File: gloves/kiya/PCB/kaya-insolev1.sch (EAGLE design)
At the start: 16 parts, among them U1 LSM9DS1, U2 MCP73832T-2ACI/OT

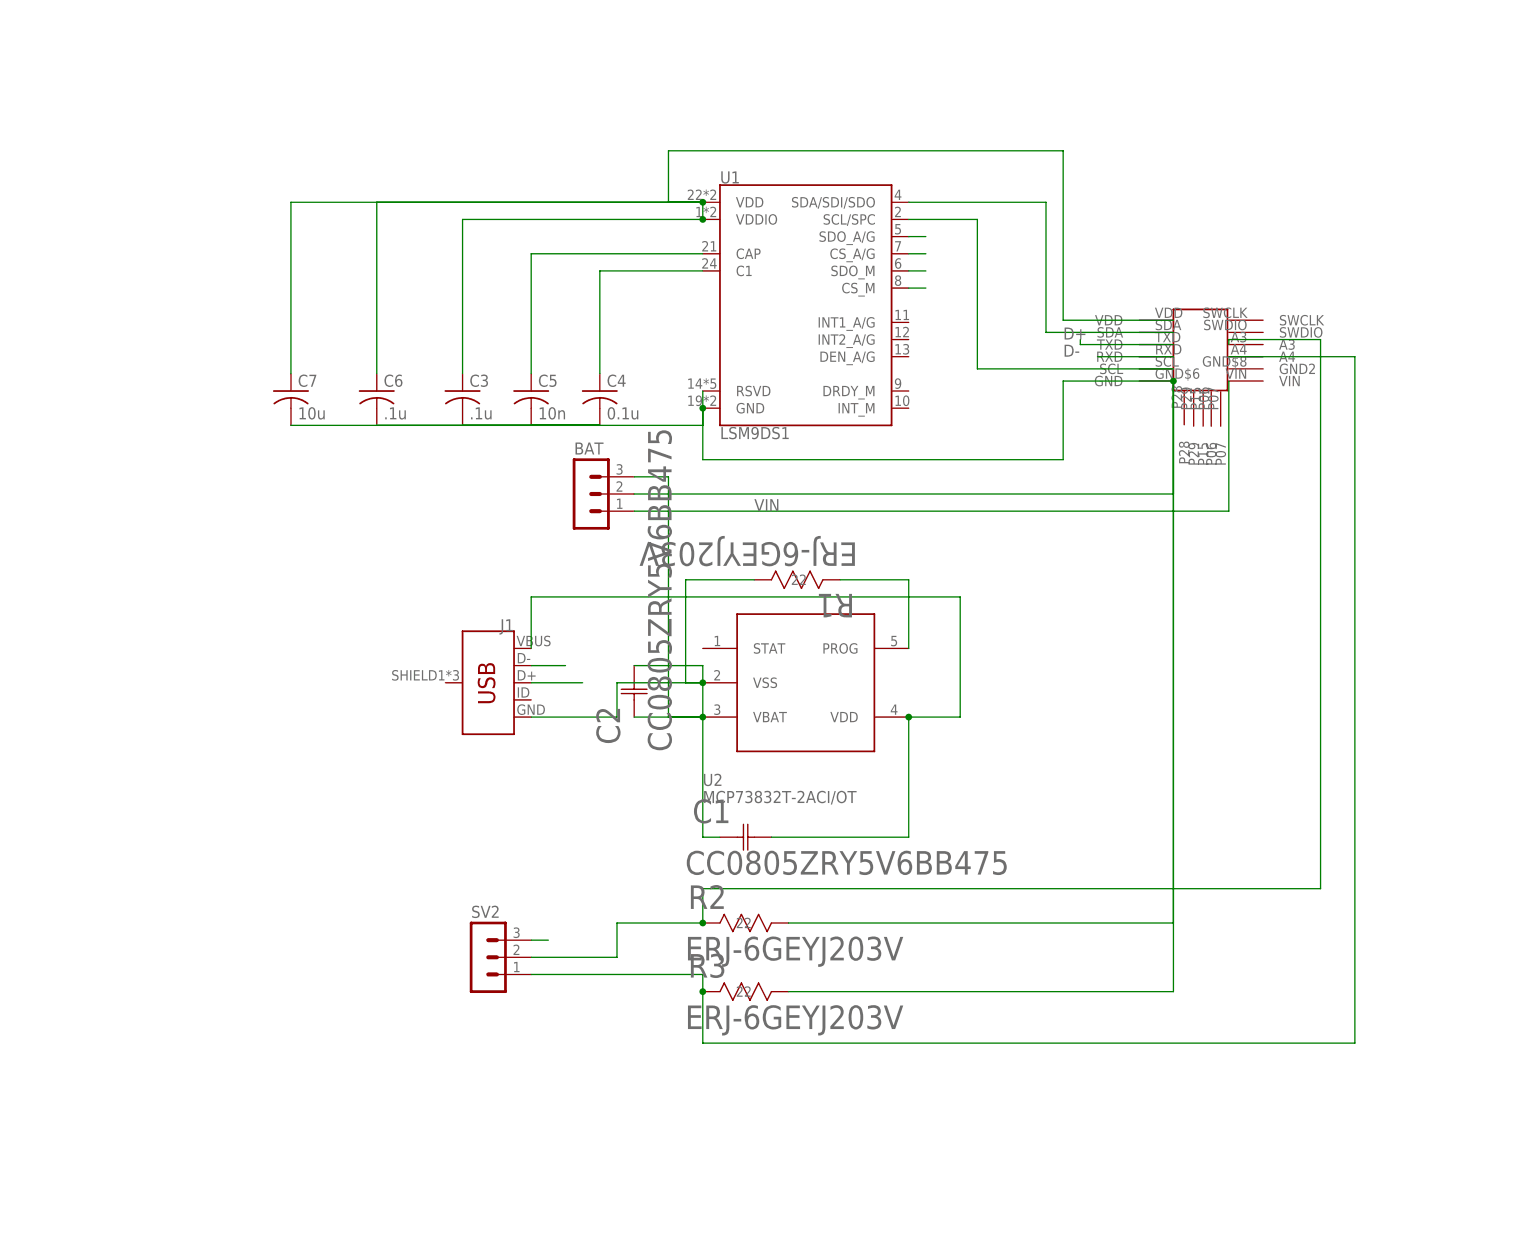
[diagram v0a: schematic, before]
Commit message: PCB v1
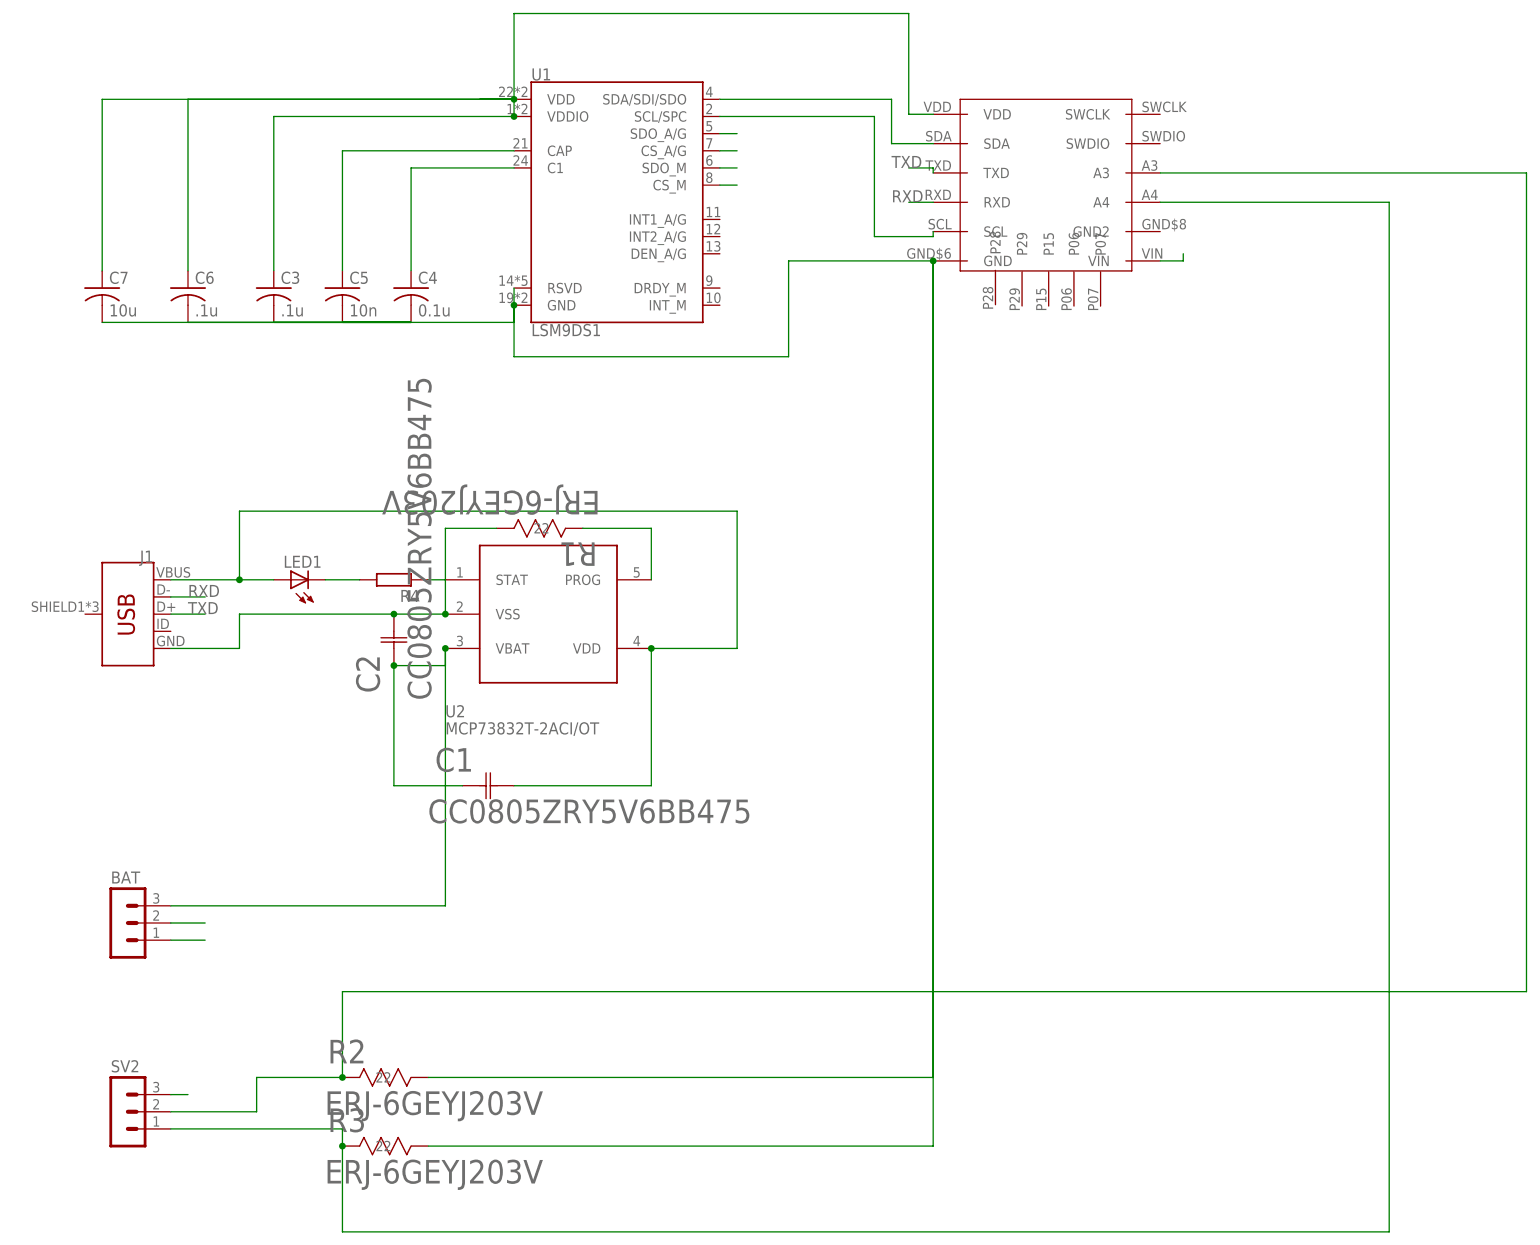
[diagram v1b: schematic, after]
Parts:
- added LED1: (no value), led:LEDCHIPLED_0603
- added R4: (no value), rcl:R-EU_R0603
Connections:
- net D+ renamed TXD
- net D- renamed RXD
- net N$2 renamed GND
- new net N$11: C2.22, J1.GND, R1.11, U2.VSS
- new net N$12: BAT.3, C1.11, C2.11, U2.VBAT
- net N$1: now also C1.22, J1.VBUS, LED1.A, U2.VDD; no longer C1.11, C2.11, C2.22, J1.GND, R1.11, U2.VSS
- net N$8: now also LED1.C, R4.2; no longer C1.22, J1.VBUS, U2.VDD
- net N$9: now also R4.1, U2.STAT; no longer BAT.3, U2.VBAT
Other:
- moved on the sheet: BAT, C1, C2, C3, C4, C5, C6, C7, J1, R1, R2, R3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
